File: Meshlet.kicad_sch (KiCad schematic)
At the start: 104 parts, among them J1 SWD, J10 Pwr Exp., J11 GPIO Exp., J12 GPS Header, J13 Thermistor Pins, J14 Ext. Notif. Header, J2 User Btn Header, J3 Batt. Header (Picoblade 1.25), J4 Batt. Header (JST-PH 2.0), J5 USB_C_Receptacle_USB2.0_16P, J6 STEMMA QT I2C, J7 Ext. Power Header, J8 I2C PINHEADER, J9 Ext. Power Header, Q1 AO3400A, SW1 RST, SW2 BOOTSEL, U1 XC6206PxxxMR, U11 INA3221, U2 USBLC6-2SC6, U3 XC6206PxxxMR, U4 RP2350_60QFN, U5 Wio-SX1262, U7 BME280, U8 W25Q32JVZP, U9 XC6206PxxxMR, Y1 12.000MHz

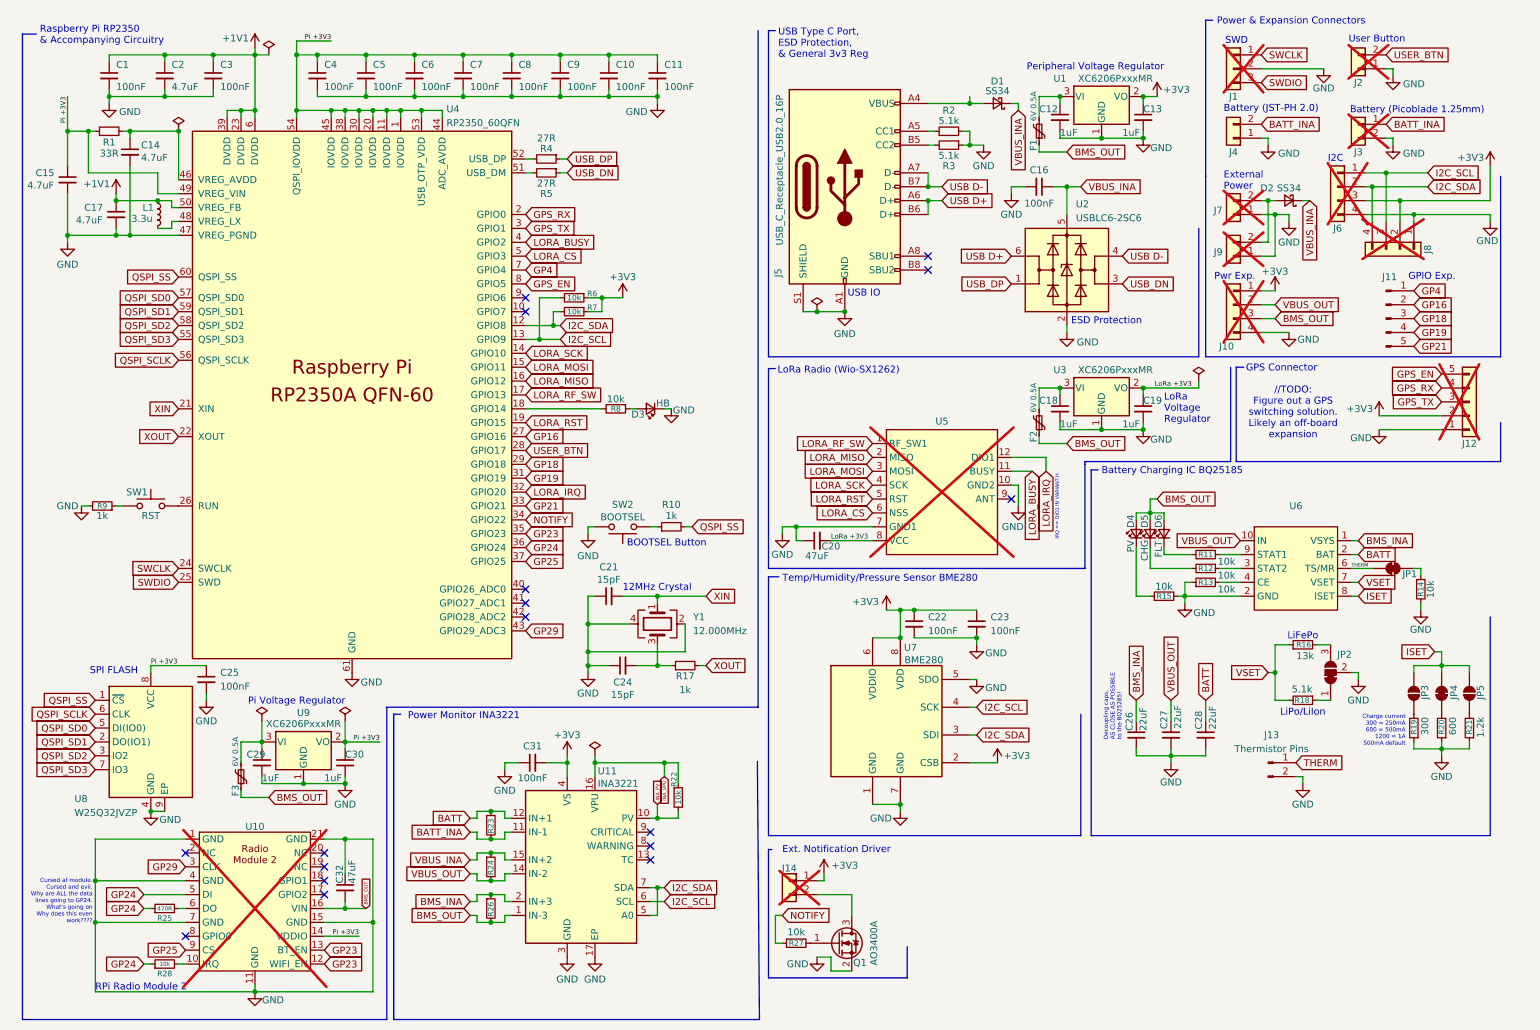
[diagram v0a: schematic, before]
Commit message: Redesign!
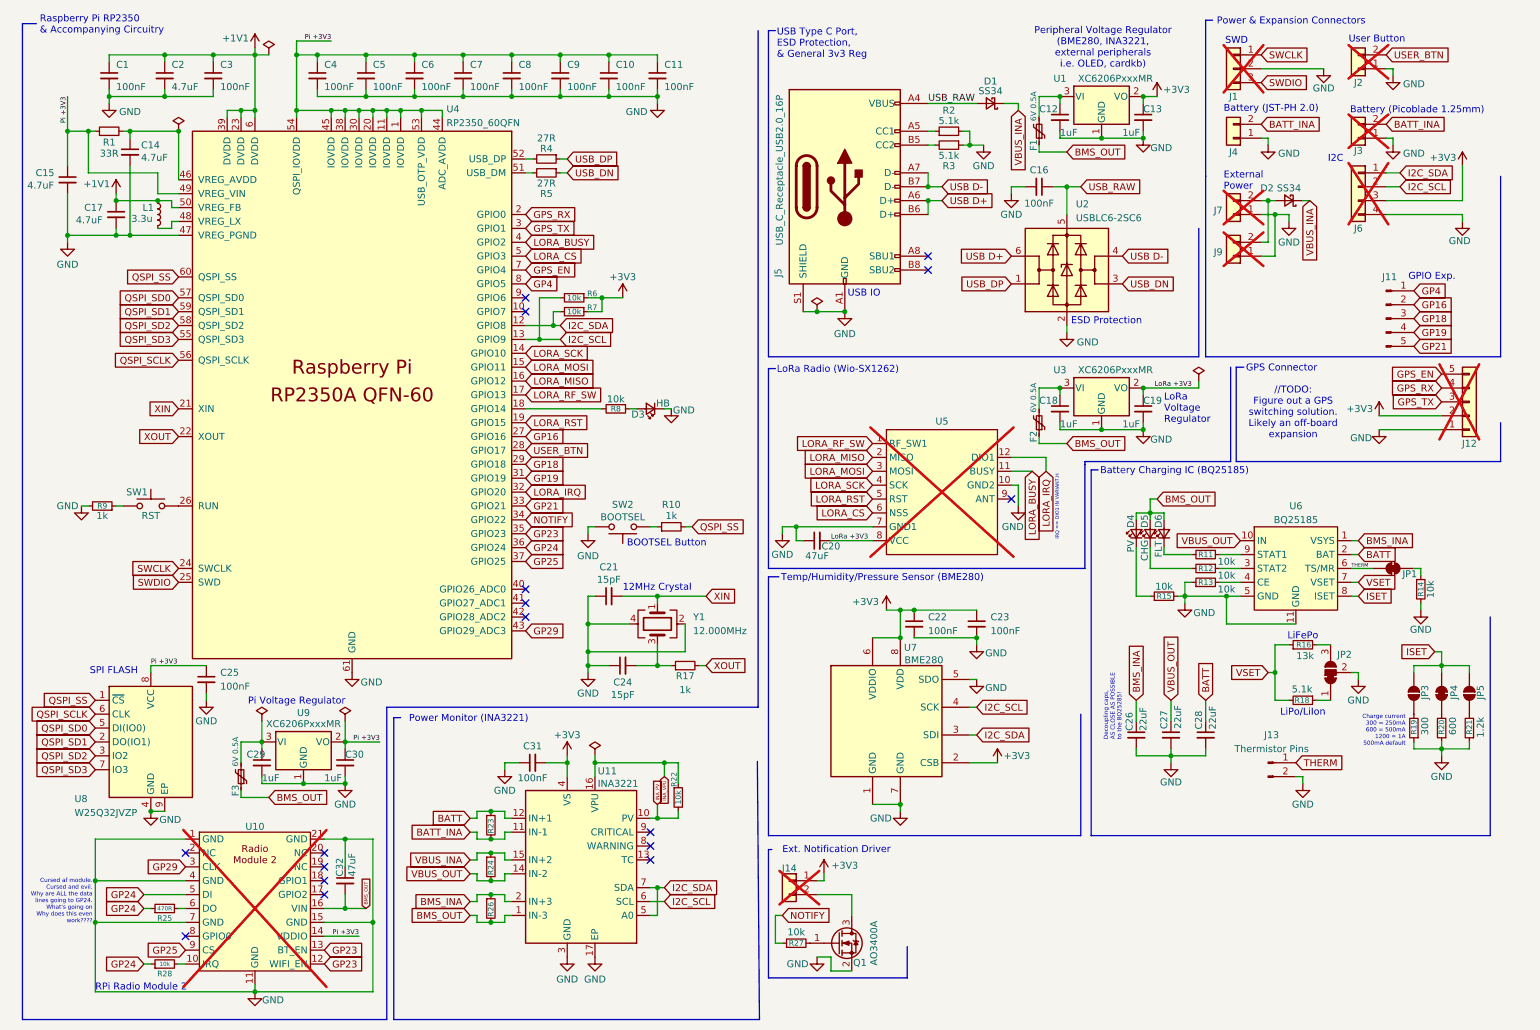
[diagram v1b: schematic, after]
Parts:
- removed J10: Pwr Exp., Connector_PinHeader_1.27mm:PinHeader_1x04_P1.27mm_Vertical, symbol Connector_Generic:Conn_01x04
- removed J8: I2C PINHEADER, Connector_PinHeader_1.27mm:PinHeader_1x04_P1.27mm_Vertical, symbol Connector_Generic:Conn_01x04
- C26, C27, C28: footprint (none) -> Capacitor_SMD:C_0402_1005Metric
- J1: footprint Connector_JST:JST_SH_SM03B-SRSS-TB_1x03-1MP_P1.00mm_Horizontal -> Connector_PinHeader_1.27mm:PinHeader_1x03_P1.27mm_Vertical
- J11: footprint (none) -> Connector_PinHeader_2.00mm:PinHeader_1x05_P2.00mm_Vertical
- J12: footprint Connector_PinHeader_1.27mm:PinHeader_1x05_P1.27mm_Vertical -> Connector_PinHeader_2.00mm:PinHeader_1x05_P2.00mm_Vertical
- J13: footprint (none) -> Connector_PinHeader_2.54mm:PinHeader_1x02_P2.54mm_Vertical
- J14, J2: footprint Connector_PinHeader_1.27mm:PinHeader_1x02_P1.27mm_Vertical -> Connector_PinHeader_2.00mm:PinHeader_1x02_P2.00mm_Vertical
- J6: footprint Connector_JST:JST_PH_S4B-PH-SM4-TB_1x04-1MP_P2.00mm_Horizontal -> Connector_PinHeader_2.00mm:PinHeader_1x04_P2.00mm_Vertical
- J7: footprint Connector_JST:JST_XH_S2B-XH-A_1x02_P2.50mm_Horizontal -> Connector_JST:JST_PH_S2B-PH-SM4-TB_1x02-1MP_P2.00mm_Horizontal
- JP1, JP4: footprint (none) -> Jumper:SolderJumper-2_P1.3mm_Bridged_RoundedPad1.0x1.5mm
- JP2: footprint (none) -> Jumper:SolderJumper-3_P1.3mm_Bridged12_RoundedPad1.0x1.5mm
- JP3, JP5: footprint (none) -> Jumper:SolderJumper-2_P1.3mm_Open_RoundedPad1.0x1.5mm
- R16, R18, R19, R20, R21: footprint (none) -> Resistor_SMD:R_0402_1005Metric
- U6: value ~ -> BQ25185; footprint (none) -> Package_DFN_QFN:Texas_DLH0010A_WSON-10-1EP_2.2x2mm_P0.4mm_EP0.9x1.5mm_ThermalVias
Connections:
- net BATT_INA: now also J3.2 (Pin_2); no longer J3.1 (Pin_1)
- net GND: now also J3.1 (Pin_1), U6.11 (GND), U6.5 (GND); no longer J3.2 (Pin_2), U6.2 (BAT)
- net GP4: now also U4.8 (GPIO5); no longer U4.7 (GPIO4)
- net GPS_EN: now also U4.7 (GPIO4); no longer U4.8 (GPIO5)
- net I2C_SCL: now also J6.2 (Pin_2); no longer J6.1 (Pin_1)
- net I2C_SDA: now also J6.1 (Pin_1); no longer J6.2 (Pin_2)
- net VBUS_INA: no longer C16.1, U2.5 (VBUS)
- net USB_RAW: now reaches D1.2 (A), J5.A4 (VBUS), J5.A9 (VBUS), J5.B4 (VBUS), J5.B9 (VBUS)
- net USB_RAW: now also C16.1, U2.5 (VBUS)
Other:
- note added: "Battery Charging IC (BQ25185)"
- note added: "Peripheral Voltage Regulator (BME280, INA3221, external peripherals i.e. OLED, cardkb)"
- note added: "Power Monitor (INA3221)"
- note added: "Temp/Humidity/Pressure Sensor (BME280)"
- note removed: "Battery Charging IC BQ25185"
- note removed: "Peripheral Voltage Regulator"
- note removed: "Power Monitor INA3221"
- note removed: "Pwr Exp."
- note removed: "Temp/Humidity/Pressure Sensor BME280"
- moved on the sheet: C32, D1, J3, J6
